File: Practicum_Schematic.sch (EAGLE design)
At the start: 25 parts, among them U1 ATMEGA328P-MU

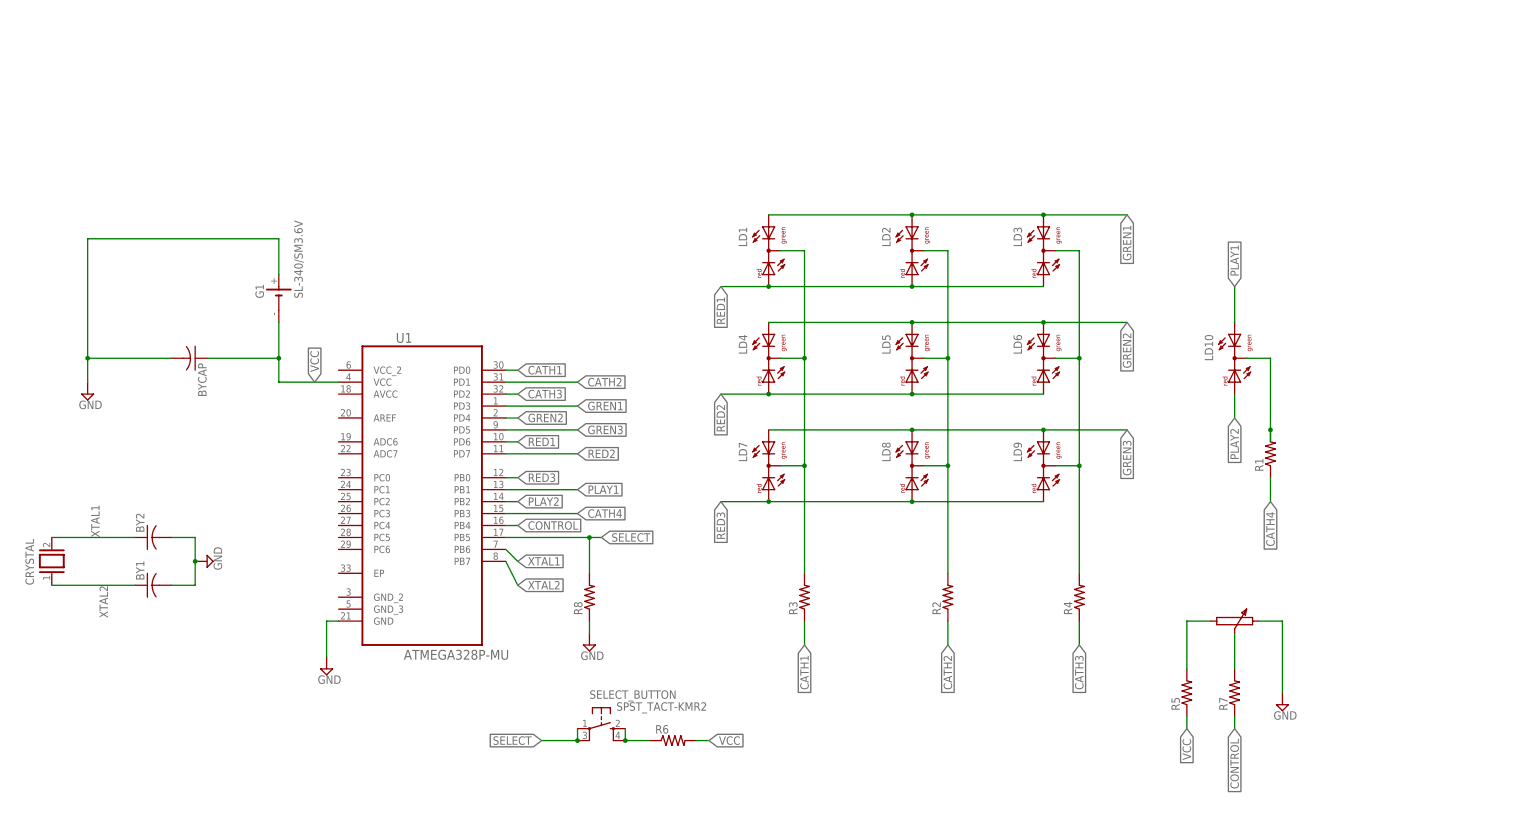
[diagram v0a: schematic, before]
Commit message: newer version ELC error free
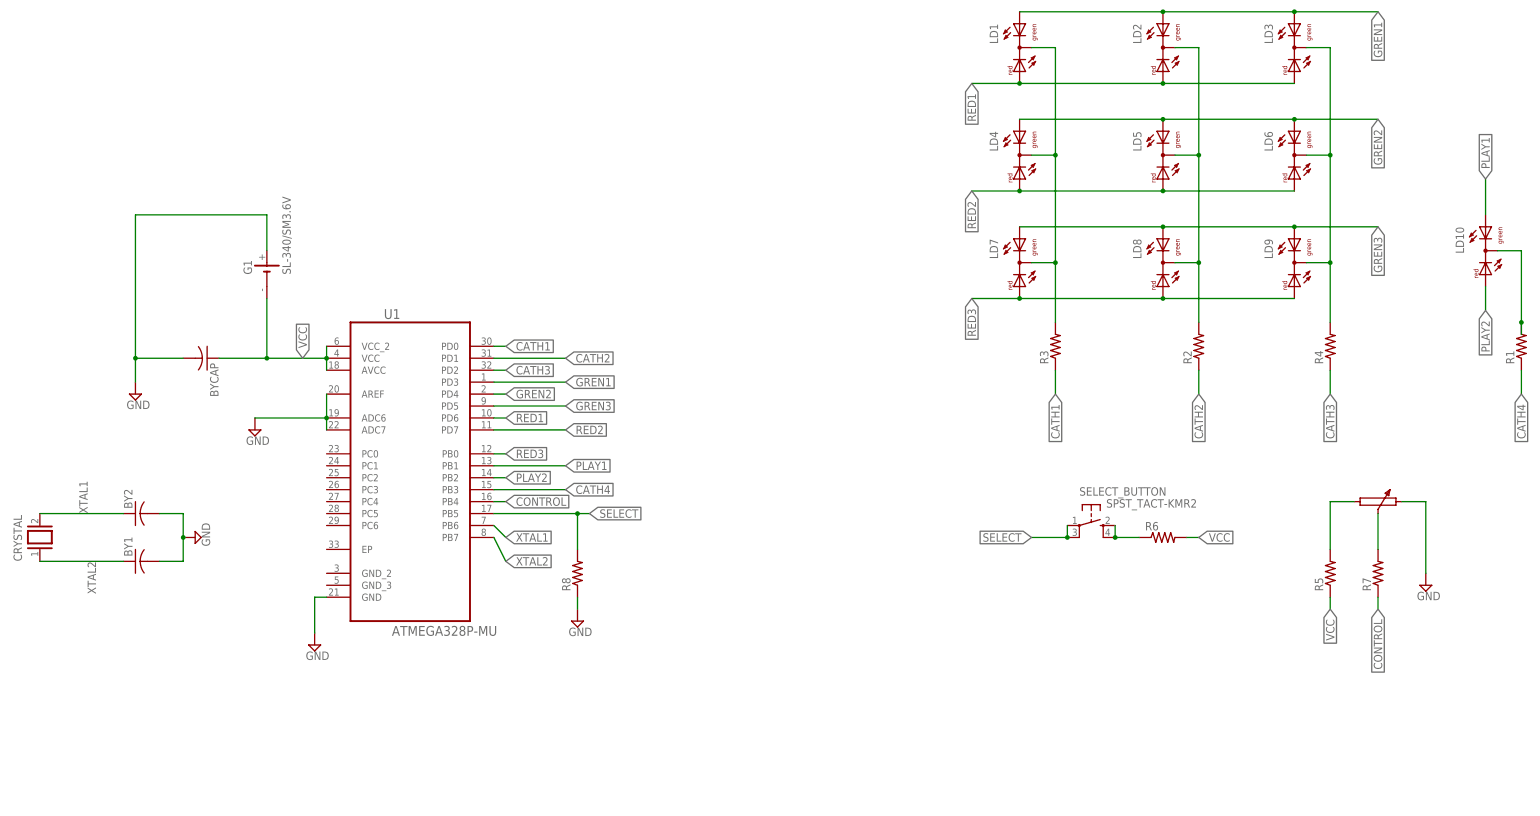
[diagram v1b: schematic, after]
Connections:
- net GND: now also U1.ADC6, U1.ADC7, U1.AREF
- net VCC: now also U1.AVCC, U1.VCC_2
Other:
- moved on the sheet: BY1, BY2, BYCAP, CRYSTAL, G1, LD1, LD10, LD2, LD3, LD4, LD5, LD6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
